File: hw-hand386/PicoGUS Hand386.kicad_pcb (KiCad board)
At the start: 4 copper layers, 29.2 x 75.2 mm, 53 parts, among them J1 AudioJack3, J3 Bus_ISA_8bit, J5 AudioJack3, J6 UART_TX, U1 Pico, U10 PCM5100, U2 SN74CB3T3245, U3 SN74CB3T3257, U4 SN74CB3T3257, U5 74AHC14, U6 74LVC00, U7 74LVC1G00, U8 APS6404L-3SQN-SN, U9 74LVC1G06

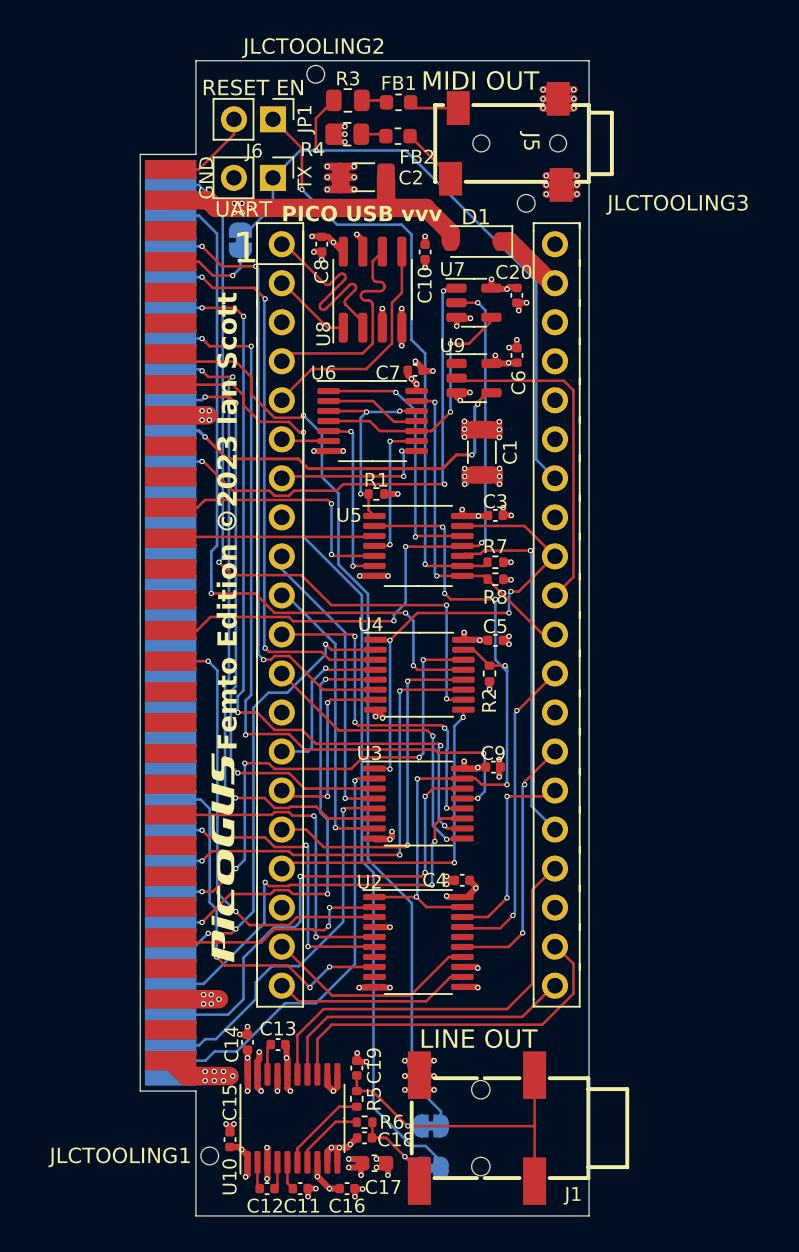
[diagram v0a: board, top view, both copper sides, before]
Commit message: v1.3 of Femto edition submitted to JLCPCB 2022-09-26
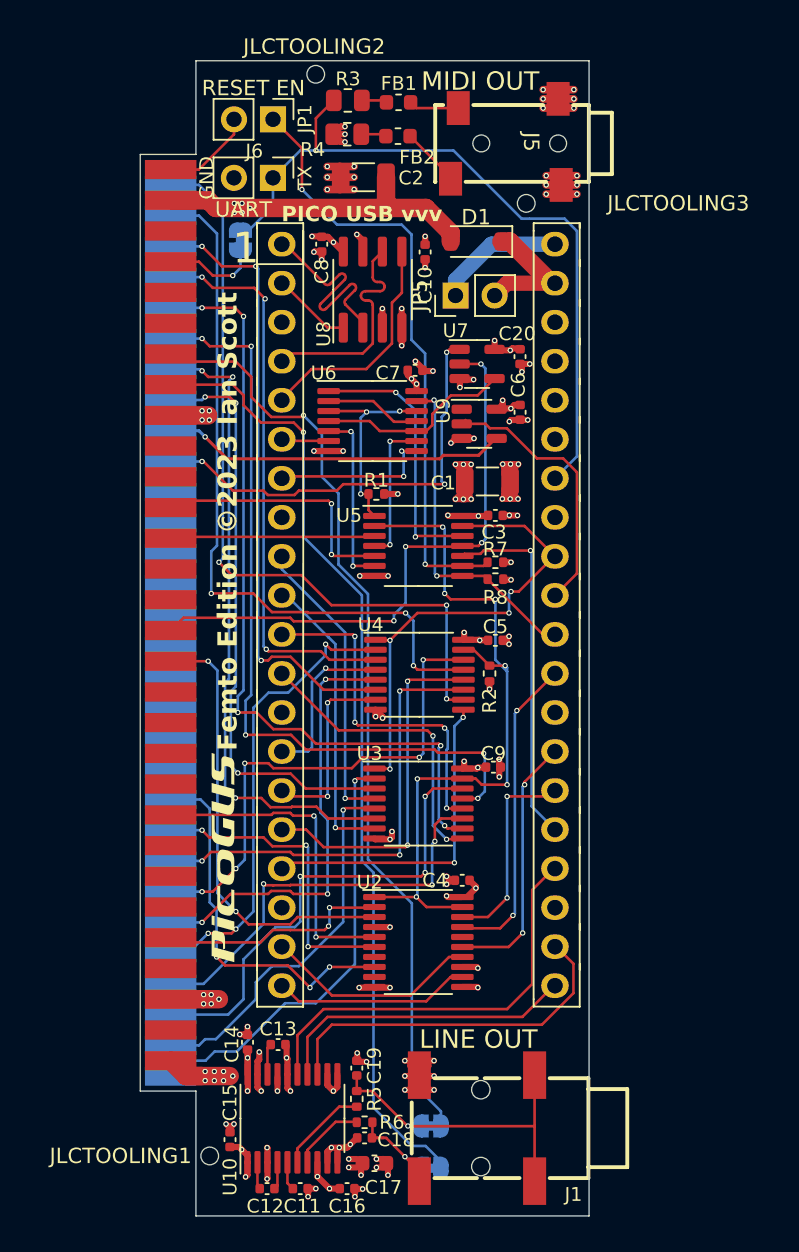
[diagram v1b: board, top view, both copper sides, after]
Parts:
- added JP5: Jumper_2_Open, Connector_PinHeader_2.54mm:PinHeader_1x02_P2.54mm_Vertical, F.Cu at (136.6, 73.7)
- moved C20 3.99 mm to (140.8, 77.7)
- moved U7 3.99 mm to (138.0, 78.2)
- moved C6 3.71 mm to (140.8, 81.3), turned to -90 degrees
- moved U9 2.99 mm to (138.1, 82.0)
- moved C1 1.93 mm to (138.7, 85.8), turned to 180 degrees
- moved REF** 0.70 mm to (133.6, 123.2)
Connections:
- U1 pad 40: unconnected-(U1-VBUS-Pad40) -> Net-(JP5-A)
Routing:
- net Net-(JP5-A): track 0.00 -> 8.44 mm
- net UART_TX: track 42.5 -> 47.2 mm
- net /VSYS: track 4.57 -> 8.83 mm
- net DACK: track 42.2 -> 38.1 mm
- net Net-(U6-Pad10): track 16.8 -> 12.9 mm, vias 2 -> 0
- net AEN: track 32.9 -> 29.1 mm
- net ~{RI/OCHRDY}: track 21.5 -> 17.8 mm
- net I/OCHRDY: track 25.4 -> 22.5 mm, vias 3 -> 1
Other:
- board text added: "Femto Edition v1.3 ©2023 Ian Scott CERN-OHL-P v2 polpo.org/picogus"
- board text removed: "Femto Edition ©2023 Ian Scott CERN-OHL-P v2 polpo.org/picogus"
- board text removed: "v1.2"
